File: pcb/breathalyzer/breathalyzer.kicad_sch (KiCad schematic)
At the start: 8 parts, among them U1 STM32F030K6Tx, U2 TLV73325PDBV

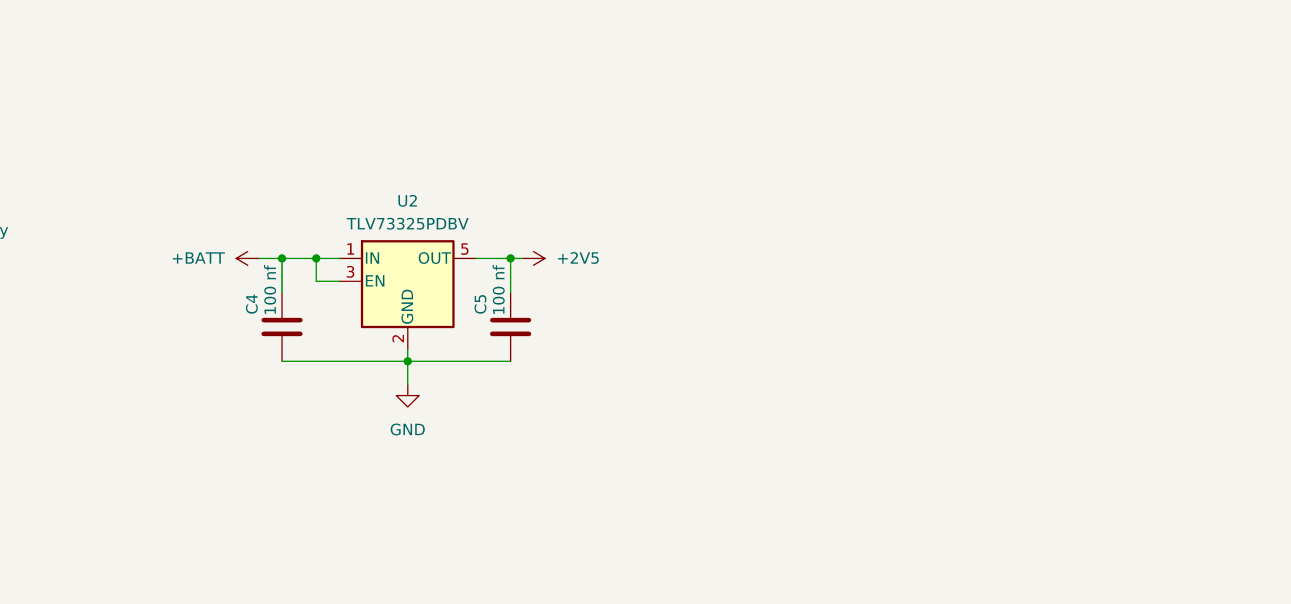
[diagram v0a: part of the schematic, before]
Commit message: voltage reference
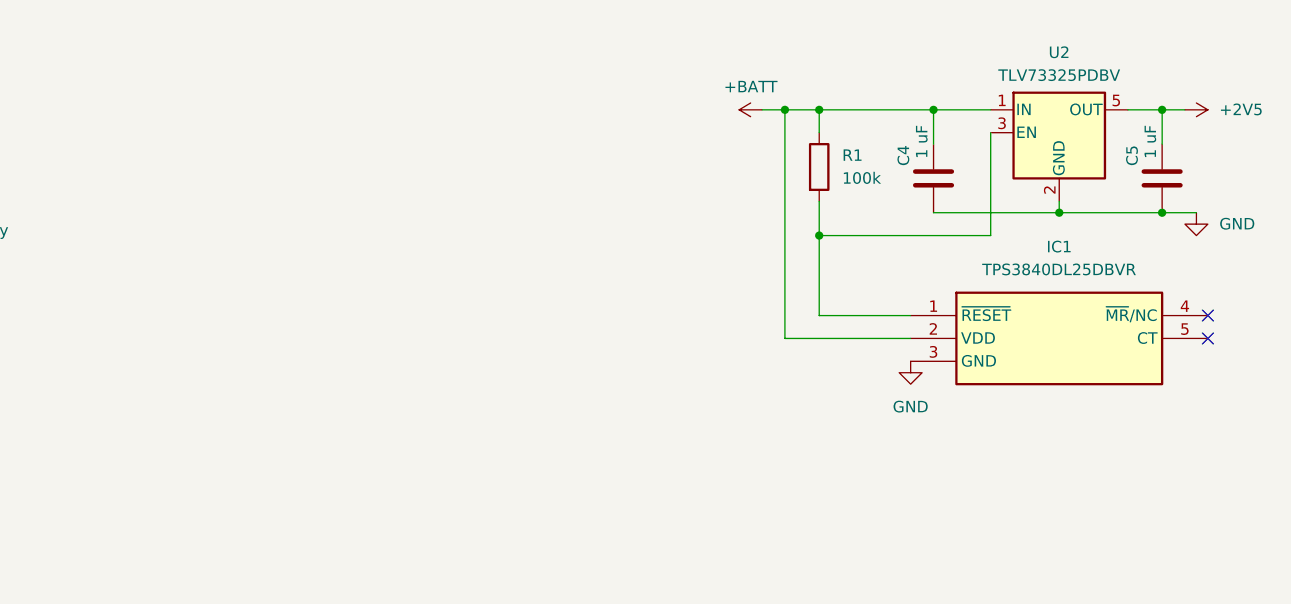
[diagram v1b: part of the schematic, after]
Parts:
- added IC1: TPS3840DL25DBVR, SOT95P280X145-5N, symbol breathalyzer:TPS3840DL25DBVR
- added R1: 100k, Resistor_SMD:R_0402_1005Metric, symbol Device:R
- C1: footprint (none) -> Capacitor_SMD:C_01005_0402Metric
- C2, C3: footprint (none) -> Capacitor_SMD:C_0402_1005Metric
- C4, C5: value 100 nf -> 1 uF; footprint (none) -> Capacitor_SMD:C_0603_1608Metric
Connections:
- net +BATT: now also IC1.2 (VDD), R1.1; no longer U2.3 (EN)
- net GND: now also IC1.3 (GND)
- new net: IC1.1 (~{RESET}), R1.2, U2.3 (EN)
- no-connect marks 0 -> 2
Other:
- moved on the sheet: C4, U2
